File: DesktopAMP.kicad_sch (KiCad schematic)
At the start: 40 parts, among them U1 PCM5222

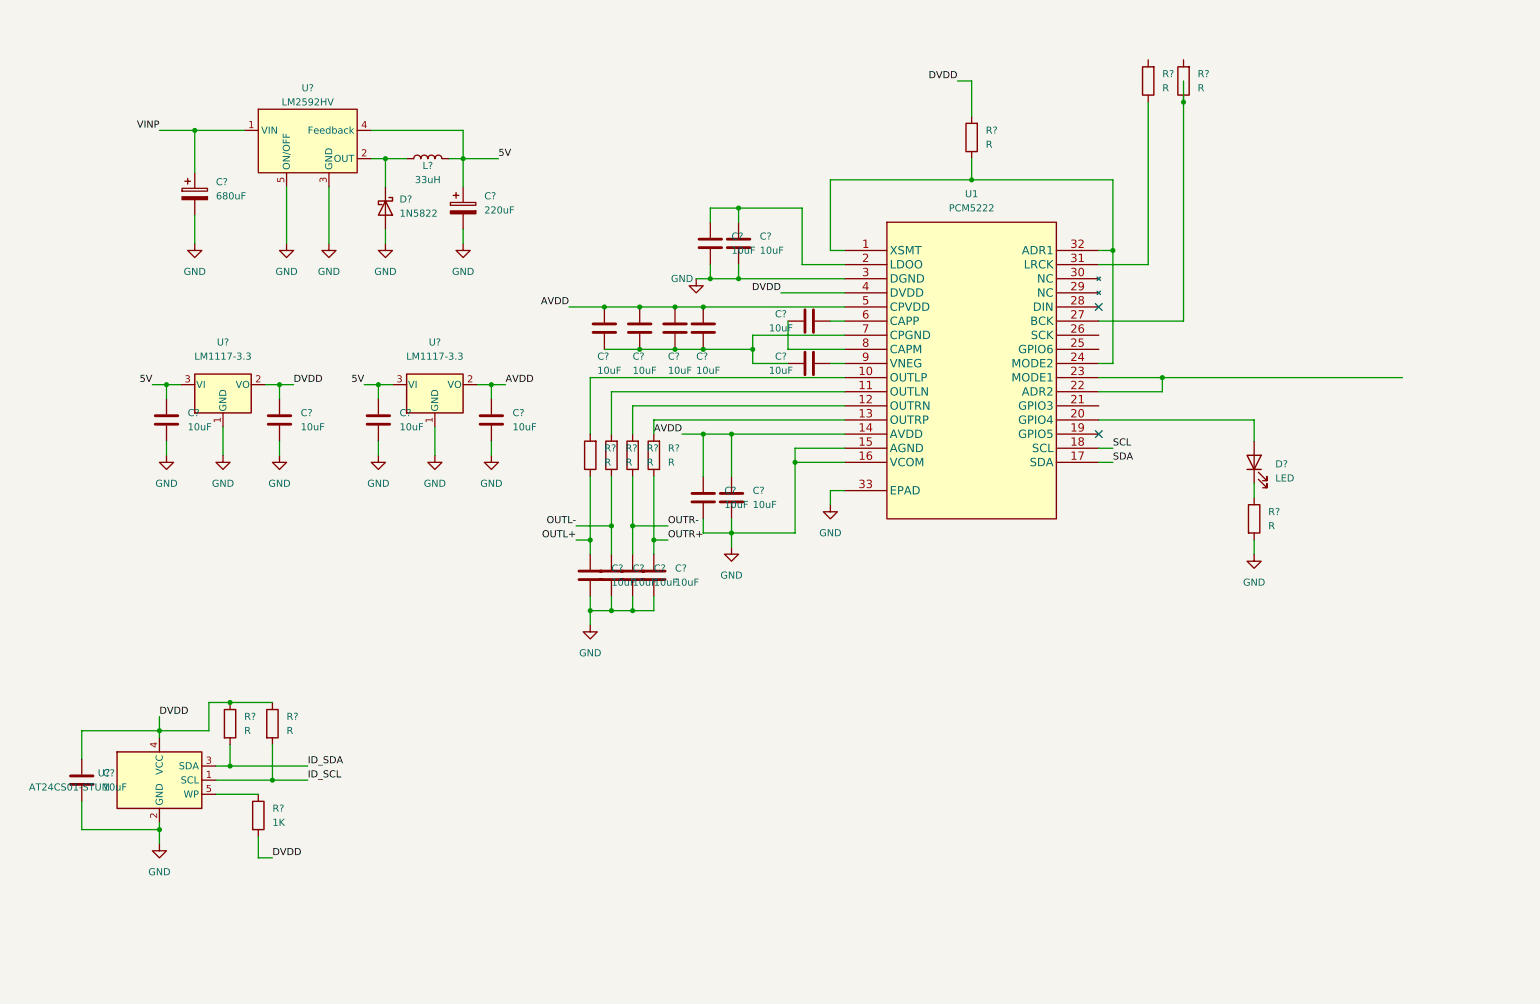
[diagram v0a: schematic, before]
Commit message: WIP
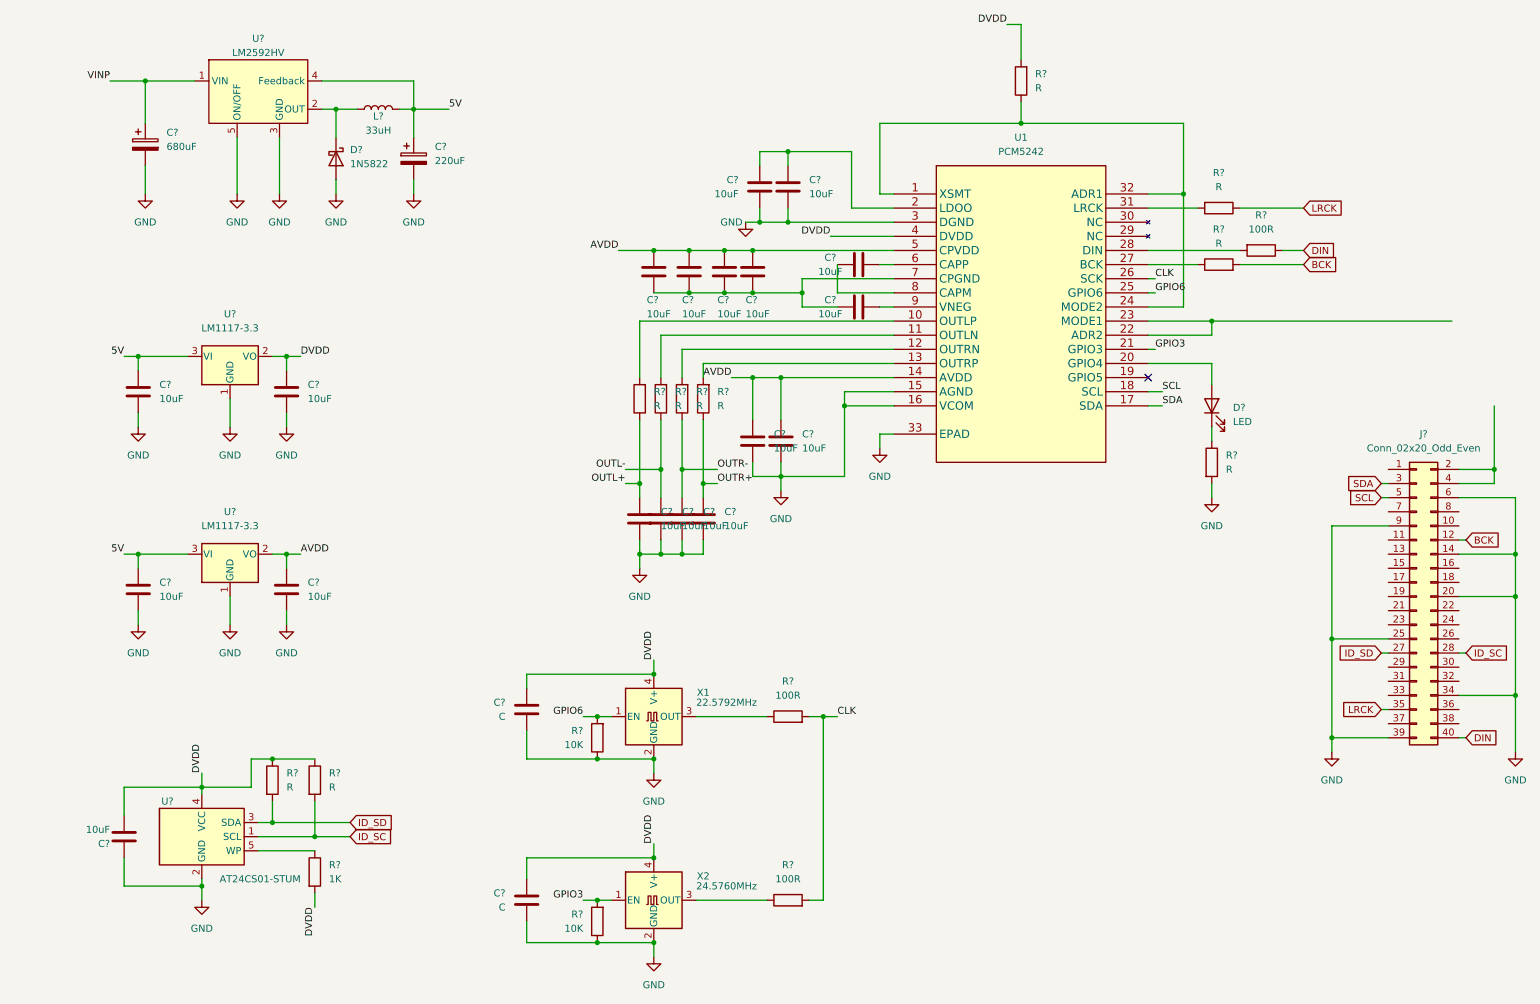
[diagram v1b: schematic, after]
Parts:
- removed C?: 10uF, symbol Device:C
- added C? (x2): C, symbol Device:C
- added C?: 10uF, symbol Device:C
- added J?: Conn_02x20_Odd_Even, symbol Connector_Generic:Conn_02x20_Odd_Even
- added R? (x3): 100R, symbol Device:R
- added R? (x2): 10K, symbol Device:R
- added X1: 22.5792MHz, Oscillator:Oscillator_SMD_EuroQuartz_XO53-4Pin_5.0x3.2mm, symbol Oscillator:XO53
- added X2: 24.5760MHz, Oscillator:Oscillator_SMD_EuroQuartz_XO53-4Pin_5.0x3.2mm, symbol Oscillator:XO53
- U1: value PCM5222 -> PCM5242
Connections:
- net 5V: now also C?.1
- net DVDD: now also C?.2, C?.2, C?.2, X1.4 (V+), X2.4 (V+); no longer C?.1
- net GND: now also C?.1, C?.1, C?.1, C?.2, J?.14 (Pin_14), J?.20 (Pin_20), J?.25 (Pin_25), J?.34 (Pin_34), J?.39 (Pin_39), J?.6 (Pin_6), J?.9 (Pin_9), R?.1, R?.1, X1.2 (GND), X2.2 (GND); no longer C?.2
- net SCL: now also J?.5 (Pin_5)
- net SDA: now also J?.3 (Pin_3)
- net GPIO3: now reaches U1.21 (GPIO3)
- net GPIO3: now also R?.2, X2.1 (EN)
- net GPIO6: now reaches U1.25 (GPIO6)
- net GPIO6: now also R?.2, X1.1 (EN)
- net CLK: now reaches U1.26 (SCK)
- net CLK: now also R?.2, R?.2
- net at U1.28 (DIN): now also R?.2
- net at U1.31 (LRCK): now also R?.2; no longer R?.1
- net BCK: now reaches R?.2
- net BCK: now also J?.12 (Pin_12)
- net ID_SCL renamed ID_SC
- net ID_SC: now also J?.28 (Pin_28)
- net ID_SDA renamed ID_SD
- net ID_SD: now also J?.27 (Pin_27)
- new net: R?.1, X1.3 (OUT)
- new net: J?.2 (Pin_2), J?.4 (Pin_4)
- new net: R?.1, X2.3 (OUT)
- new net DIN: J?.40 (Pin_40), R?.1
- new net LRCK: J?.35 (Pin_35), R?.1
- no-connect marks 2 -> 1
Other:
- moved on the sheet: C?, D?, L?, R?, U1, U?
